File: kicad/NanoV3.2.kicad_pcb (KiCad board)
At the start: 2 copper layers, 43.2 x 17.8 mm, 51 parts, among them IC1 FT232RL, IC2 LM1117IMPX-5.0, IC3 ATMEGA328P-AU, J1 Strip15pin, J2 Strip15pin, J3 USB-mini-90 -SMD, J4 ICSP, SW1 157SW, Y1 CSTCE16M0V53-R0

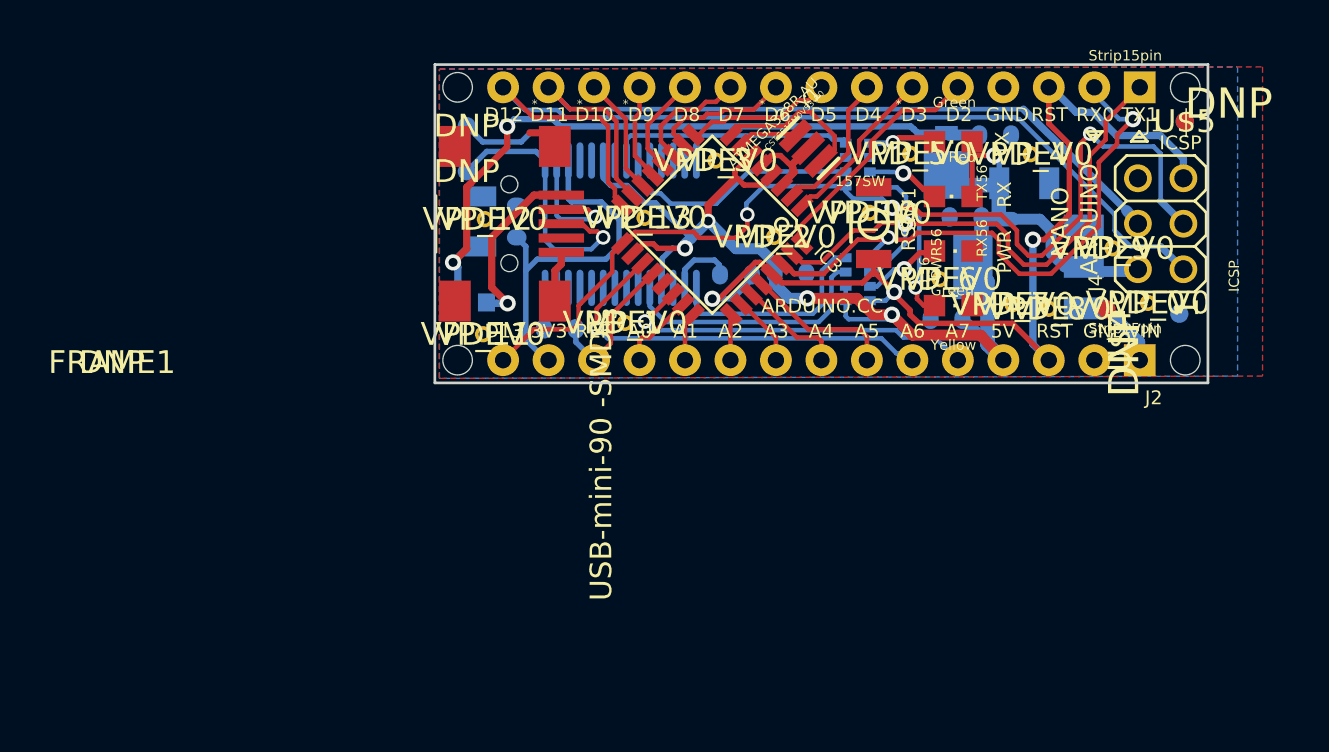
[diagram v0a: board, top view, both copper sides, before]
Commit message: updated schematic, not workable yet
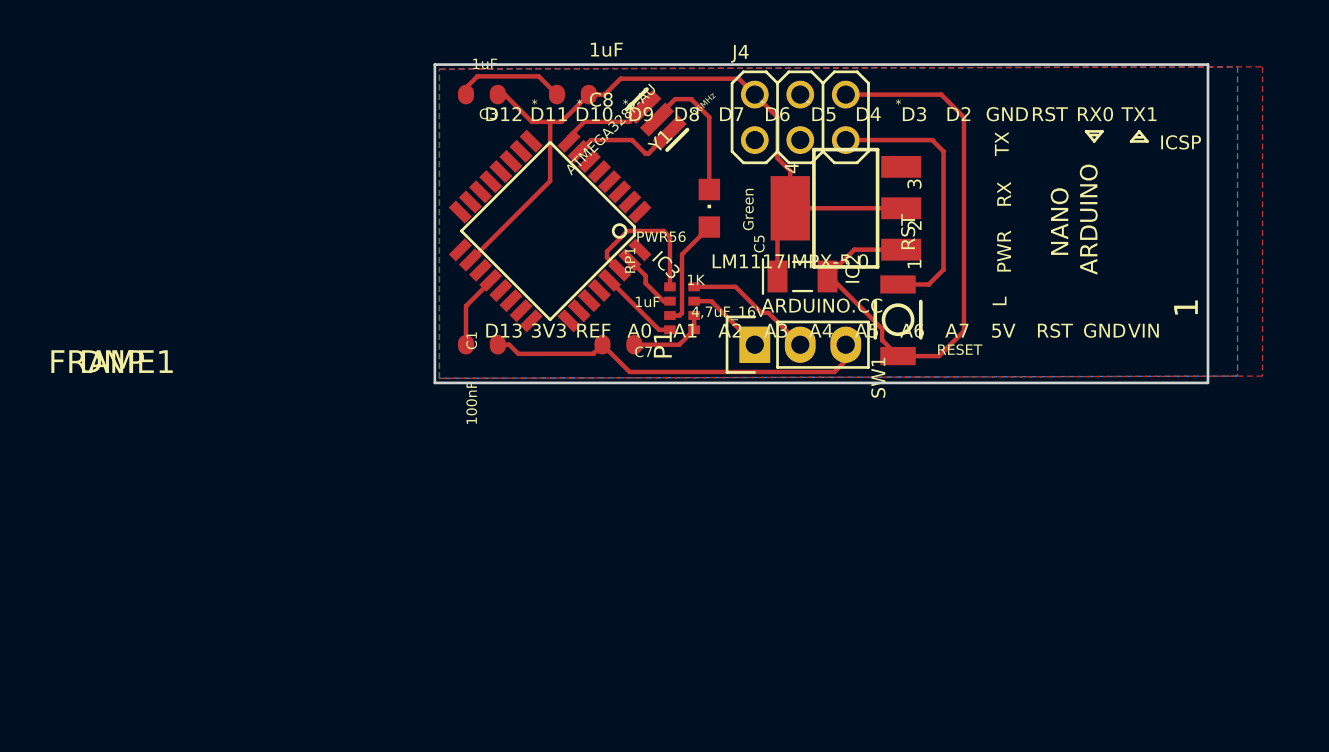
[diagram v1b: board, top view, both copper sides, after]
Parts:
- removed @HOLE0, @HOLE1, @HOLE2, @HOLE3: , 
- removed C2: 4,7uF_16V, TAN-A
- removed C4, C6, C9: 100nF, C0603-ROUND
- removed D+56, D-56: DNP, TP-1.00MM
- removed D1: SS1P3L, DO220AAL
- removed F1: MFFSMF050, 0603-1608X90N
- removed IC1: FT232RL, SSOP28
- removed J1, J2: Strip15pin, HEAD15-NOSS
- removed J3: USB-mini-90 -SMD, USB-MINI-B_2
- removed L56: Yellow, CHIPLED_0805
- removed RP2: 1K, CAY16
- removed RX56: Red, CHIPLED_0805
- removed TX56: Green, CHIPLED_0805
- removed U$4, U$5, U$53, U$54: DNP, FD-1-1.5
- removed VP_0, VP_1, VP_10, VP_11, VP_12, VP_13, VP_2, VP_3, VP_4, VP_5, VP_6, VP_7, VP_8, VP_9: VPDEV0, VPAC0
- added P1: CONN_01X03, Pin_Headers:Pin_Header_Straight_1x03, F.Cu at (144.8, 111.8)
- C1, C3, C5, C7, C8, IC2, RP1: moved to F.Cu
- J4: value ICSP -> ~
- SW1: value 157SW -> RESET
- Y1: value CSTCE16M0V53-R0 -> 16MHz
- moved C8 24.3 mm to (134.6, 97.8)
- moved J4 21.0 mm to (147.3, 99.1), turned to 0 degrees
- moved C7 20.7 mm to (137.2, 111.8)
- moved C3 19.9 mm to (129.5, 97.8), turned to 180 degrees
- moved PWR56 13.8 mm to (142.2, 104.1), turned to 0 degrees
- moved C5 13.4 mm to (146.1, 108.0)
- moved IC2 10.7 mm to (149.9, 104.1), turned to 90 degrees
- moved RP1 9.95 mm to (140.7, 109.7)
- moved SW1 9.52 mm to (152.8, 112.4), turned to 90 degrees
- moved IC3 9.06 mm to (133.3, 105.4)
- moved Y1 8.60 mm to (139.3, 99.2), turned to 135 degrees
- moved C1 4.45 mm to (129.5, 111.8), turned to 0 degrees
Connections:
- net AREF renamed /AREF
- net D0/RX renamed /D0/RX
- net D1/TX renamed /D1/TX
- net D11/MOSI renamed /D11/MOSI
- net D12/MISO renamed /D12/MISO
- net D13/SCK renamed /D13/SCK
- net N$1 renamed /N$1
- net N$2 renamed /N$2
- net N$3 renamed /N$3
- net RESET renamed /RESET
- IC2 pad 3: VIN -> (no net)
- IC3 pad 1: D3 -> (no net)
- IC3 pad 10: D6 -> (no net)
- IC3 pad 11: D7 -> (no net)
- IC3 pad 12: D8 -> (no net)
- IC3 pad 13: D9 -> (no net)
- IC3 pad 14: D10 -> (no net)
- IC3 pad 19: A6 -> (no net)
- IC3 pad 2: D4 -> (no net)
- IC3 pad 22: A7 -> (no net)
- IC3 pad 23: A0 -> (no net)
- IC3 pad 24: A1 -> (no net)
- IC3 pad 25: A2 -> (no net)
- IC3 pad 26: A3 -> (no net)
- IC3 pad 27: A4 -> (no net)
- IC3 pad 28: A5 -> (no net)
- IC3 pad 32: D2 -> (no net)
- IC3 pad 9: D5 -> (no net)
- RP1 pad 7: TX -> /TX
- RP1 pad 8: RX -> Net-(P1-Pad2)
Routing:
- net COM: track 10.4 -> 69.9 mm
- net /D13/SCK: track 55.6 -> 0.00 mm, vias 3 -> 0
- net /D12/MISO: track 54.3 -> 0.00 mm
- net /D11/MOSI: track 45.6 -> 0.00 mm
- net VUSB: track 40.3 -> 0.00 mm, vias 2 -> 0
- net /RESET: track 56.7 -> 19.7 mm, vias 3 -> 0
- net +5V: track 84.0 -> 47.9 mm, vias 5 -> 0
- net /D1/TX: track 33.0 -> 3.44 mm, vias 1 -> 0
- net /D0/RX: track 33.4 -> 8.33 mm, vias 2 -> 0
- net A6: track 23.6 -> 0.00 mm, vias 1 -> 0
- net A7: track 21.0 -> 0.00 mm, vias 1 -> 0
- net 3V3: track 20.4 -> 0.00 mm
- net N$5: track 16.0 -> 0.00 mm, vias 1 -> 0
- net TX: track 14.5 -> 0.00 mm
- net N$6: track 14.5 -> 0.00 mm, vias 1 -> 0
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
